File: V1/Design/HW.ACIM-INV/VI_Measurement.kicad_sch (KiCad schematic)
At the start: 45 parts, among them Q1 20V/1A, U18 OP-1CH, U19 OP-1CH, U4 CMP-1CH, U6 ISEN 50mV/V, U8 OP-1CH

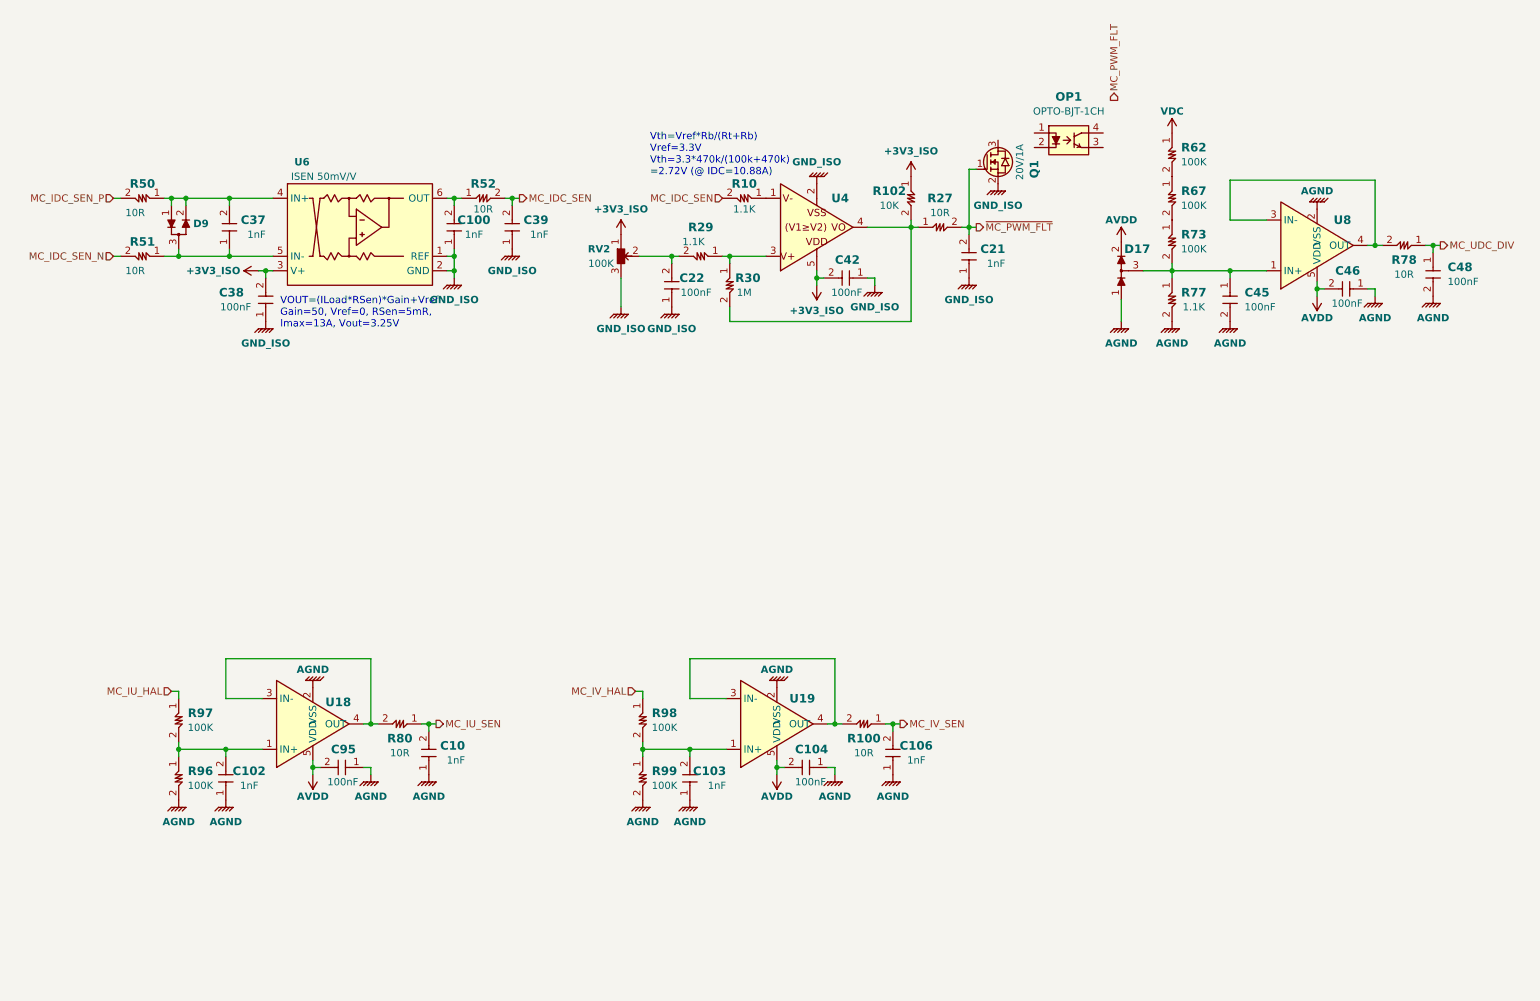
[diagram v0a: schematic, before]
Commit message: V1 schematic update 12
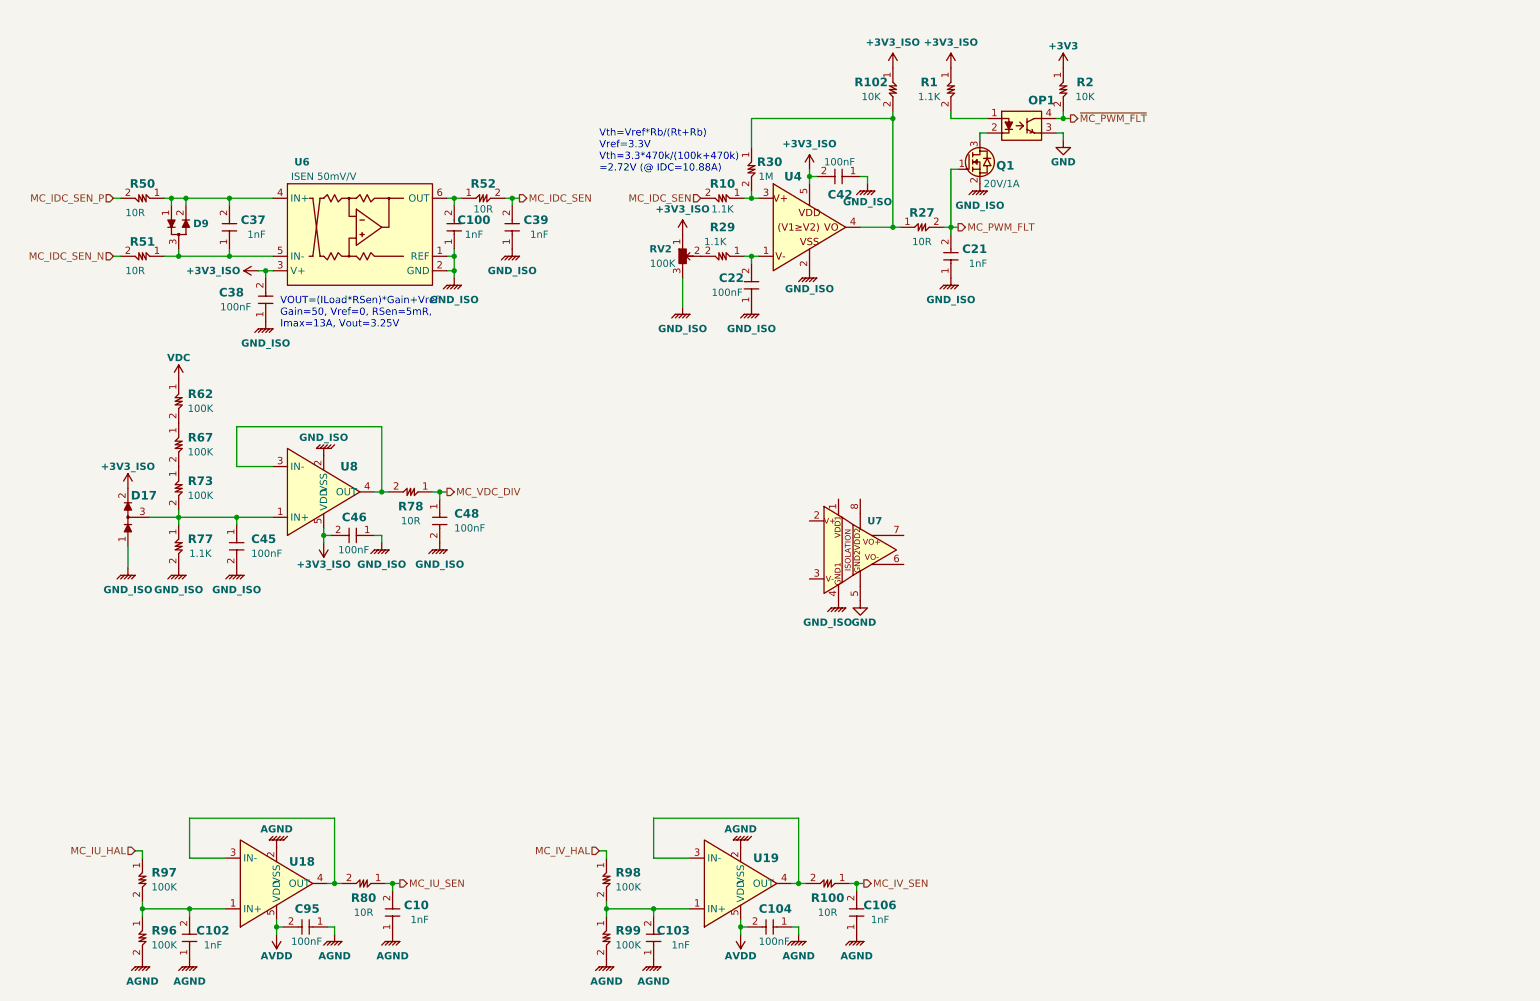
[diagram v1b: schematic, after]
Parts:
- added R1: 1.1K, SAMPI:RES0603, symbol SAMPI:RES
- added R2: 10K, SAMPI:RES0603, symbol SAMPI:RES
- added U7: ISO OPAMP 1-CH, symbol SAMPI:ISO-OPAMP
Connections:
- net +3V3_ISO: now also C46.2, D17.2 (K2), U8.5 (VDD), R1.1
- net AGND: no longer C45.2, C46.1, C48.2, D17.1 (A1), R77.2, U8.2 (VSS)
- net AVDD: no longer C46.2, D17.2 (K2), U8.5 (VDD)
- net GND_ISO: now also C45.2, C46.1, C48.2, D17.1 (A1), R77.2, U8.2 (VSS), U7.4 (GND1)
- net MC_PWM_FLT: now also C21.2, Q1.1 (G), R27.2
- net ~{MC_PWM_FLT}: now also OP1.4 (C), R2.2; no longer C21.2, Q1.1 (G), R27.2
- net at R29.2, RV2.2 (WIPER): no longer C22.2
- net at R102.2, R27.1, U4.4 (VOUT): now also R30.1; no longer R30.2
- net at OP1.1 (A): now also R1.2
- net at OP1.2 (K): now also Q1.3 (D)
- net GND: now reaches OP1.3 (E)
- net GND: now also U7.5 (GND2)
- net at R10.1: now also R30.2, U4.3 (VIN+); no longer U4.1 (VIN-)
- net MC_UDC_DIV renamed MC_VDC_DIV
- new net: C22.2, R29.1, U4.1 (VIN-)
- new net +3V3: R2.1
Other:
- moved on the sheet: C10, C102, C103, C104, C106, C21, C22, C42, C45, C46, C48, C95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
